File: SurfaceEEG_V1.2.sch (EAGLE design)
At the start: 52 parts, among them IC1 LMV602, IC2 TSZ124IQ4T, U1 MCP4442-103E/ST

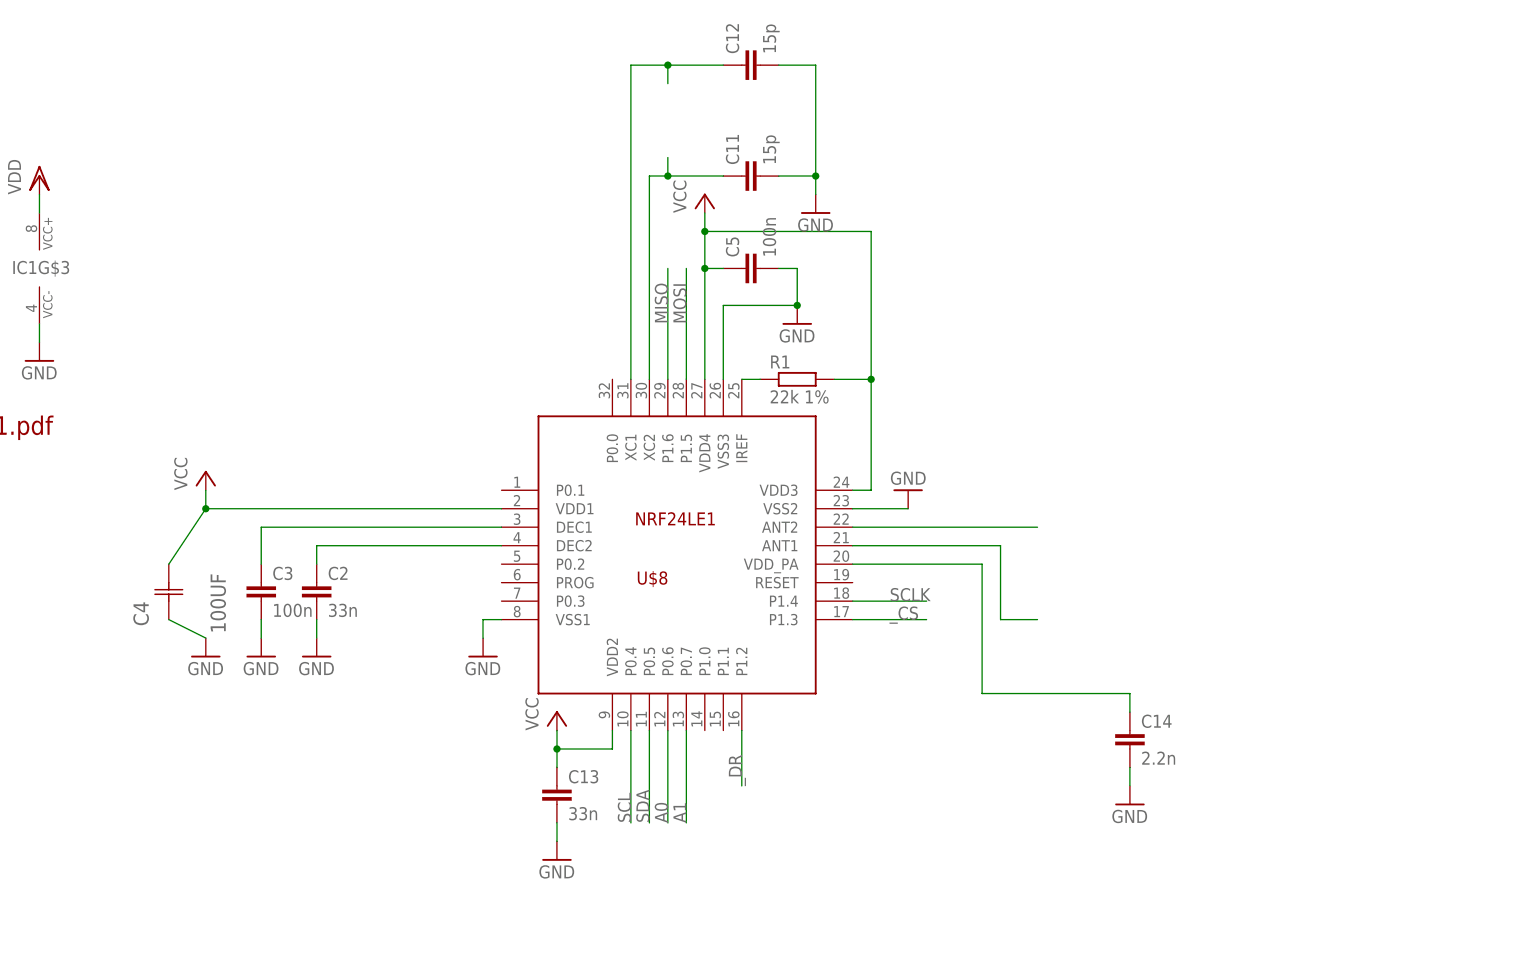
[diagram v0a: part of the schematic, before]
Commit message: Added RF antenna schematics
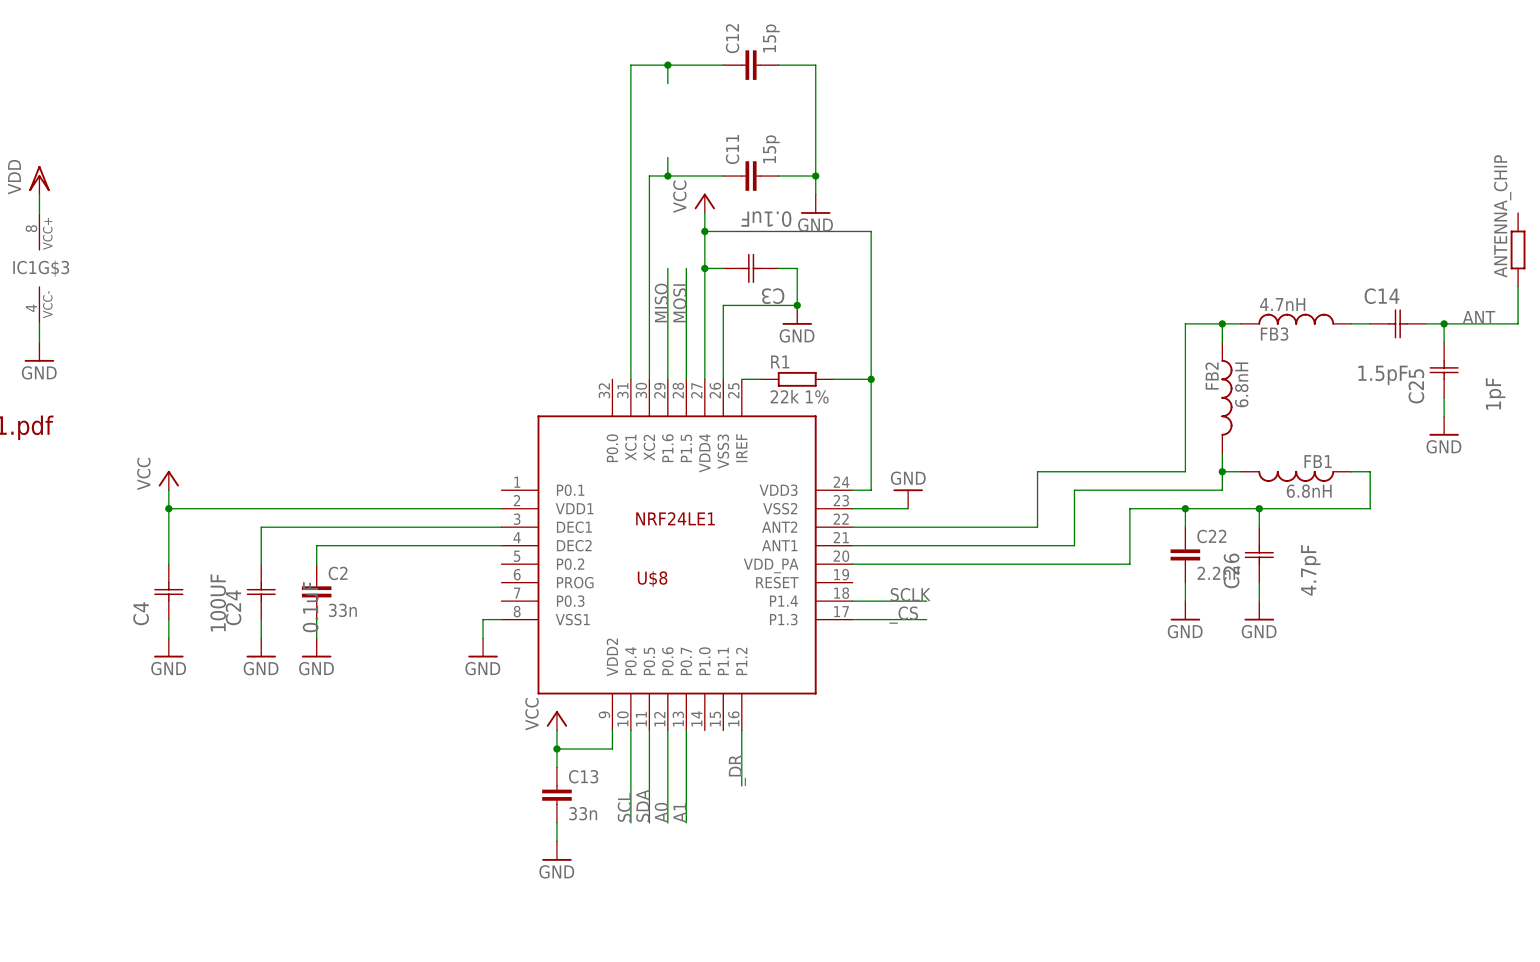
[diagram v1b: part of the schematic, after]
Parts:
- removed C5: 100n, ELL-i-Passives:C0402
- added ANTENNA_CHIP: (no value), ELL-i-Passives:R0805
- added C22: 2.2nF, ELL-i-Passives:C0603
- added C24: 0.1uF, (manufact)-capacitors-AVX-element14:04023C104KAT2A
- added C25: 1pF, (manufact)-capacitors-AVX-element14:UQCL2A1R0BAT2A/500
- added C26: 4.7pF, (manufact)-capacitors-AVX-element14:UQCL2A4R7CAT2A/500
- added FB1, FB2: 6.8nH, ELL-i-Passives:FB0402
- added FB3: 4.7nH, ELL-i-Passives:FB0402
- C14: value 2.2n -> 1.5pF; device ELL-i-Passives:C0402 -> (manufact)-capacitors-AVX-element14:UQCL2A1R5BAT2A/500
- C3: value 100n -> 0.1uF; device ELL-i-Passives:C0402 -> (manufact)-capacitors-AVX-element14:04023C104KAT2A
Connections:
- removed net N$6: U$8.ANT2
- removed net N$8: C14.1, U$8.VDD_PA
- new net ANT: ANTENNA_CHIP.1, C14.C2, C25.C2
- new net N$1: FB2.1, FB3.1, U$8.ANT2
- new net N$22: C14.C1, FB3.2
- new net N$4: C22.1, C26.C2, FB1.1, U$8.VDD_PA
- net GND: now also C22.2, C24.C1, C25.C1, C26.C1, C3.C1; no longer C14.2, C3.2, C5.2
- net N$2: now also C24.C2; no longer C3.1
- net N$7: now also FB1.2, FB2.2
- net VCC: now also C3.C2; no longer C5.1
